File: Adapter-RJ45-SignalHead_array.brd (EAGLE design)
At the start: 119.4 x 106.7 mm, 25 parts

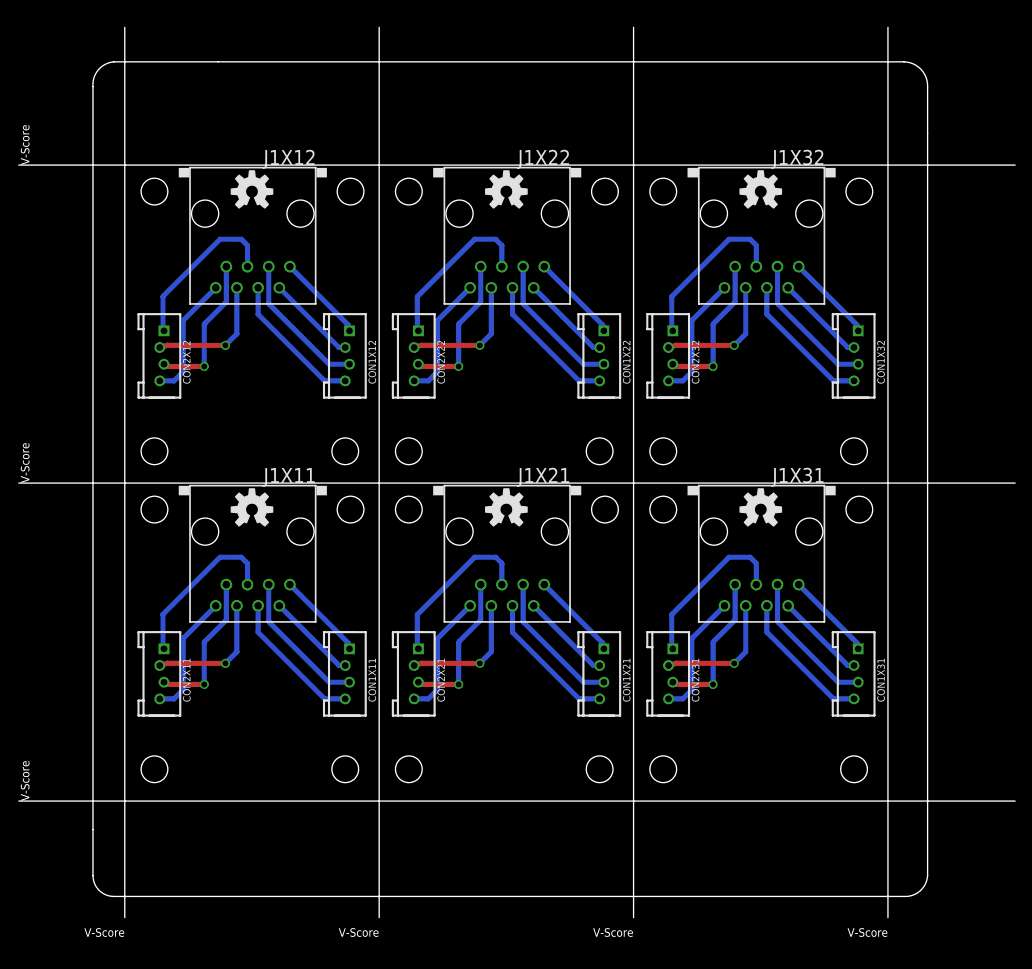
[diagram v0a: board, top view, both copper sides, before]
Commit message: V3.2 - added CUT-R
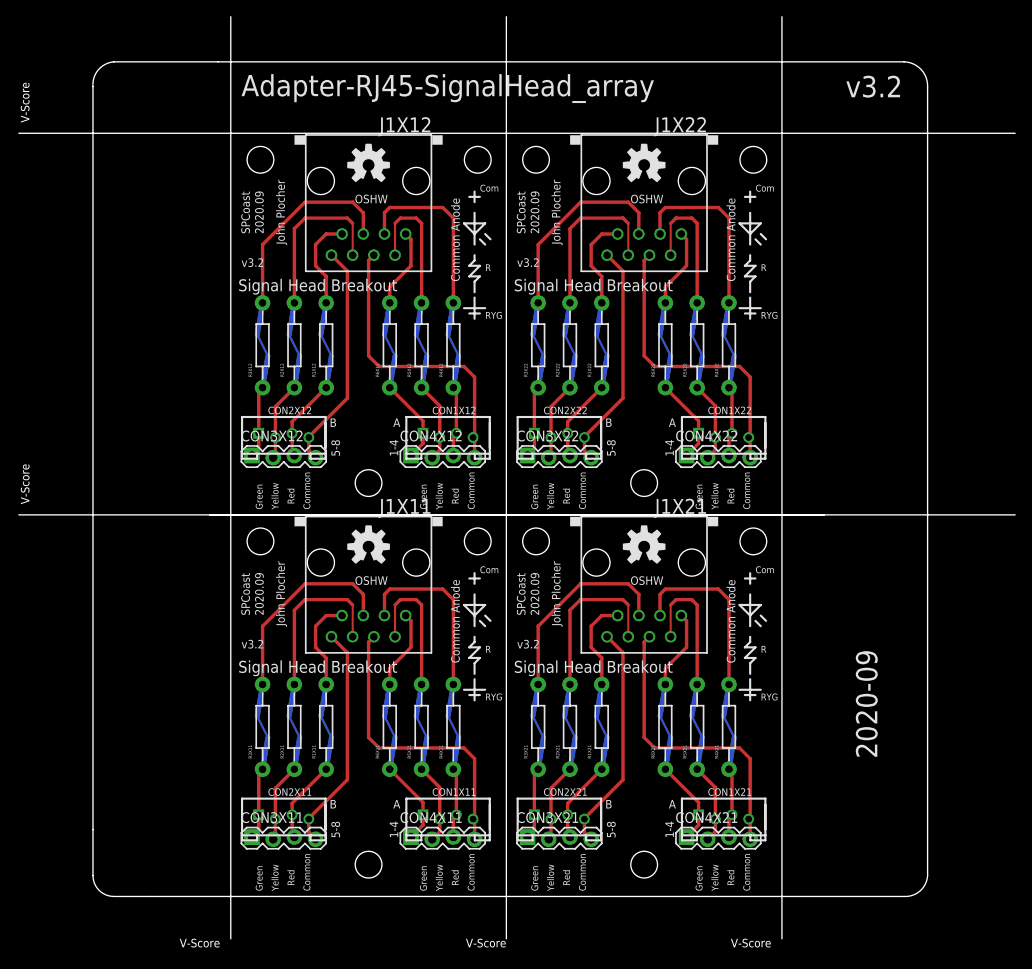
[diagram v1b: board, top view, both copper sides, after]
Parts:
- removed CON1X31, CON1X32, CON2X31, CON2X32: (no value), SPCoast:4P-2.0
- removed J1X31, J1X32: (no value), SPCoast:RJ45-NO-SHIELD
- removed U$1X31, U$1X32: (no value), SPCoast:OSHW-LOGO-M
- added CON3X11, CON3X12, CON3X21, CON3X22, CON4X11, CON4X12, CON4X21, CON4X22: (no value), SPCoast:1X04_LOCK
- added R1X11, R1X12, R1X21, R1X22, R2X11, R2X12, R2X21, R2X22, R3X11, R3X12, R3X21, R3X22, R4X11, R4X12, R4X21, R4X22, R5X11, R5X12, R5X21, R5X22, R6X11, R6X12, R6X21, R6X22: (no value), SPCoast:CUT-R
- U$1X11, U$1X12, U$1X21, U$1X22: value (none) -> DOC-OSHW-LOGO-M
- moved CON2X21 24.2 mm to (55.9, 9.53), turned to 0 degrees
- moved CON2X11 22.5 mm to (22.9, 9.53), turned to 0 degrees
- moved CON1X21 22.5 mm to (75.6, 9.53), turned to 0 degrees
- moved CON1X11 21.0 mm to (42.5, 9.53), turned to 0 degrees
- moved CON2X22 19.6 mm to (55.9, 55.2), turned to 0 degrees
- moved CON1X22 17.4 mm to (75.6, 55.2), turned to 0 degrees
- moved CON2X12 17.4 mm to (22.9, 55.2), turned to 0 degrees
- moved U$1X21 17.1 mm to (66.0, 41.9)
- moved J1X22 16.9 mm to (66.0, 85.7)
- moved J1X21 16.8 mm to (66.0, 40.0)
- moved U$1X22 16.8 mm to (66.0, 87.6)
- moved CON1X12 15.4 mm to (42.5, 55.2), turned to 0 degrees
- moved U$1X11 14.7 mm to (33.0, 41.9)
- moved J1X12 14.4 mm to (33.0, 85.7)
- moved J1X11 14.4 mm to (33.0, 40.0)
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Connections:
- removed net L5X11: CON2X11.1, J1X11.5
- removed net L5X12: CON2X12.1, J1X12.5
- removed net L5X21: CON2X21.1, J1X21.5
- removed net L5X22: CON2X22.1, J1X22.5
- removed net L5X31: CON2X31.1, J1X31.5
- removed net L5X32: CON2X32.1, J1X32.5
- removed net L6X11: CON2X11.2, J1X11.6
- removed net L6X12: CON2X12.2, J1X12.6
- removed net L6X21: CON2X21.2, J1X21.6
- removed net L6X22: CON2X22.2, J1X22.6
- removed net L6X31: CON2X31.2, J1X31.6
- removed net L6X32: CON2X32.2, J1X32.6
- removed net L7X11: CON2X11.3, J1X11.7
- removed net L7X12: CON2X12.3, J1X12.7
- removed net L7X21: CON2X21.3, J1X21.7
- removed net L7X22: CON2X22.3, J1X22.7
- removed net L7X31: CON2X31.3, J1X31.7
- removed net L7X32: CON2X32.3, J1X32.7
- removed net L8X11: CON2X11.4, J1X11.8
- removed net L8X12: CON2X12.4, J1X12.8
- removed net L8X21: CON2X21.4, J1X21.8
- removed net L8X22: CON2X22.4, J1X22.8
- removed net L8X31: CON2X31.4, J1X31.8
- removed net L8X32: CON2X32.4, J1X32.8
- removed net N$1X11: CON1X11.1, J1X11.1
- removed net N$1X12: CON1X12.1, J1X12.1
- removed net N$1X21: CON1X21.1, J1X21.1
- removed net N$1X22: CON1X22.1, J1X22.1
- removed net N$1X31: CON1X31.1, J1X31.1
- removed net N$1X32: CON1X32.1, J1X32.1
- removed net N$2X11: CON1X11.2, J1X11.2
- removed net N$2X12: CON1X12.2, J1X12.2
- removed net N$2X21: CON1X21.2, J1X21.2
- removed net N$2X22: CON1X22.2, J1X22.2
- removed net N$2X31: CON1X31.2, J1X31.2
- removed net N$2X32: CON1X32.2, J1X32.2
- removed net N$3X11: CON1X11.3, J1X11.3
- removed net N$3X12: CON1X12.3, J1X12.3
- removed net N$3X21: CON1X21.3, J1X21.3
- removed net N$3X22: CON1X22.3, J1X22.3
- removed net N$3X31: CON1X31.3, J1X31.3
- removed net N$3X32: CON1X32.3, J1X32.3
- removed net N$4X11: CON1X11.4, J1X11.4
- removed net N$4X12: CON1X12.4, J1X12.4
- removed net N$4X21: CON1X21.4, J1X21.4
- removed net N$4X22: CON1X22.4, J1X22.4
- removed net N$4X31: CON1X31.4, J1X31.4
- removed net N$4X32: CON1X32.4, J1X32.4
- new net A-COMMONX11: CON1X11.4, CON4X11.4, J1X11.4
- new net A-COMMONX12: CON1X12.4, CON4X12.4, J1X12.4
- new net A-COMMONX21: CON1X21.4, CON4X21.4, J1X21.4
- new net A-COMMONX22: CON1X22.4, CON4X22.4, J1X22.4
- new net AGRX11: CON1X11.1, CON4X11.1, R6X11.P2
- new net AGRX12: CON1X12.1, CON4X12.1, R6X12.P2
- new net AGRX21: CON1X21.1, CON4X21.1, R6X21.P2
- new net AGRX22: CON1X22.1, CON4X22.1, R6X22.P2
- new net AGX11: J1X11.1, R6X11.P1
- new net AGX12: J1X12.1, R6X12.P1
- new net AGX21: J1X21.1, R6X21.P1
- new net AGX22: J1X22.1, R6X22.P1
- new net ARRX11: CON1X11.3, CON4X11.3, R4X11.P2
- new net ARRX12: CON1X12.3, CON4X12.3, R4X12.P2
- new net ARRX21: CON1X21.3, CON4X21.3, R4X21.P2
- new net ARRX22: CON1X22.3, CON4X22.3, R4X22.P2
- new net ARX11: J1X11.3, R4X11.P1
- new net ARX12: J1X12.3, R4X12.P1
- new net ARX21: J1X21.3, R4X21.P1
- new net ARX22: J1X22.3, R4X22.P1
- new net AYRX11: CON1X11.2, CON4X11.2, R5X11.P2
- new net AYRX12: CON1X12.2, CON4X12.2, R5X12.P2
- new net AYRX21: CON1X21.2, CON4X21.2, R5X21.P2
- new net AYRX22: CON1X22.2, CON4X22.2, R5X22.P2
- new net AYX11: J1X11.2, R5X11.P1
- new net AYX12: J1X12.2, R5X12.P1
- new net AYX21: J1X21.2, R5X21.P1
- new net AYX22: J1X22.2, R5X22.P1
- new net B-COMMONX11: CON2X11.4, CON3X11.4, J1X11.8
- new net B-COMMONX12: CON2X12.4, CON3X12.4, J1X12.8
- new net B-COMMONX21: CON2X21.4, CON3X21.4, J1X21.8
- new net B-COMMONX22: CON2X22.4, CON3X22.4, J1X22.8
- new net BGRX11: CON2X11.1, CON3X11.1, R3X11.P2
- new net BGRX12: CON2X12.1, CON3X12.1, R3X12.P2
- new net BGRX21: CON2X21.1, CON3X21.1, R3X21.P2
- new net BGRX22: CON2X22.1, CON3X22.1, R3X22.P2
- new net BGX11: J1X11.5, R3X11.P1
- new net BGX12: J1X12.5, R3X12.P1
- new net BGX21: J1X21.5, R3X21.P1
- new net BGX22: J1X22.5, R3X22.P1
- new net BRRX11: CON2X11.3, CON3X11.3, R1X11.P2
- new net BRRX12: CON2X12.3, CON3X12.3, R1X12.P2
- new net BRRX21: CON2X21.3, CON3X21.3, R1X21.P2
- new net BRRX22: CON2X22.3, CON3X22.3, R1X22.P2
- new net BRX11: J1X11.7, R1X11.P1
- new net BRX12: J1X12.7, R1X12.P1
- new net BRX21: J1X21.7, R1X21.P1
- new net BRX22: J1X22.7, R1X22.P1
- new net BYRX11: CON2X11.2, CON3X11.2, R2X11.P2
- new net BYRX12: CON2X12.2, CON3X12.2, R2X12.P2
- new net BYRX21: CON2X21.2, CON3X21.2, R2X21.P2
- new net BYRX22: CON2X22.2, CON3X22.2, R2X22.P2
- new net BYX11: J1X11.6, R2X11.P1
- new net BYX12: J1X12.6, R2X12.P1
- new net BYX21: J1X21.6, R2X21.P1
- new net BYX22: J1X22.6, R2X22.P1
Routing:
- net A-COMMONX11: track 0.00 -> 35.9 mm
- net A-COMMONX12: track 0.00 -> 35.9 mm
- net A-COMMONX22: track 0.00 -> 35.9 mm
- net A-COMMONX21: track 0.00 -> 35.9 mm
- net B-COMMONX11: track 0.00 -> 27.3 mm
- net B-COMMONX12: track 0.00 -> 27.3 mm
- net B-COMMONX21: track 0.00 -> 27.3 mm
- net B-COMMONX22: track 0.00 -> 27.3 mm
- net BGX21: track 0.00 -> 24.2 mm
- net BGX22: track 0.00 -> 24.2 mm
- net BGX11: track 0.00 -> 24.2 mm
- net BGX12: track 0.00 -> 24.2 mm
- net ARX22: track 0.00 -> 21.7 mm
- net ARX21: track 0.00 -> 21.7 mm
- net ARX11: track 0.00 -> 21.7 mm
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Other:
- board size 119.4 x 106.7 mm -> 119.4 x 110.5 mm
- board text added: "2020-09"
- board text added: "2020.09"
- board text added: ">DRAWING_NAME"
- board text added: "CON1"
- board text added: "CON2"
- board text added: "CON3"
- board text added: "CON4"
- board text added: "Com"
- board text added: "Common"
- board text added: "Common Anode"
- board text added: "Cut traces is using resistors"
- board text added: "J1"
- board text added: "OSHW"
- board text added: "R"
- board text added: "R1"
- board text added: "R2"
- board text added: "R3"
- board text added: "R4"
- board text added: "R5"
- board text added: "R6"
- board text added: "RYG"
- board text added: "Signal Head Breakout"
- board text added: "V3.2"
- board text added: "v3.2"
- board text added: "www. SPCoast .com"
- board text removed: "+ Common +"
- board text removed: ".com"
- board text removed: "2018-01"
- board text removed: "Adapter RJ45 to Signal Head"
- board text removed: "Go Bears!"
- board text removed: "SP Coast"
- board text removed: "V3.1"
- board text removed: "v3.1"
- board text removed: "www."
